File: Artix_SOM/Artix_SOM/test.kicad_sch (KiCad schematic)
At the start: 1 part

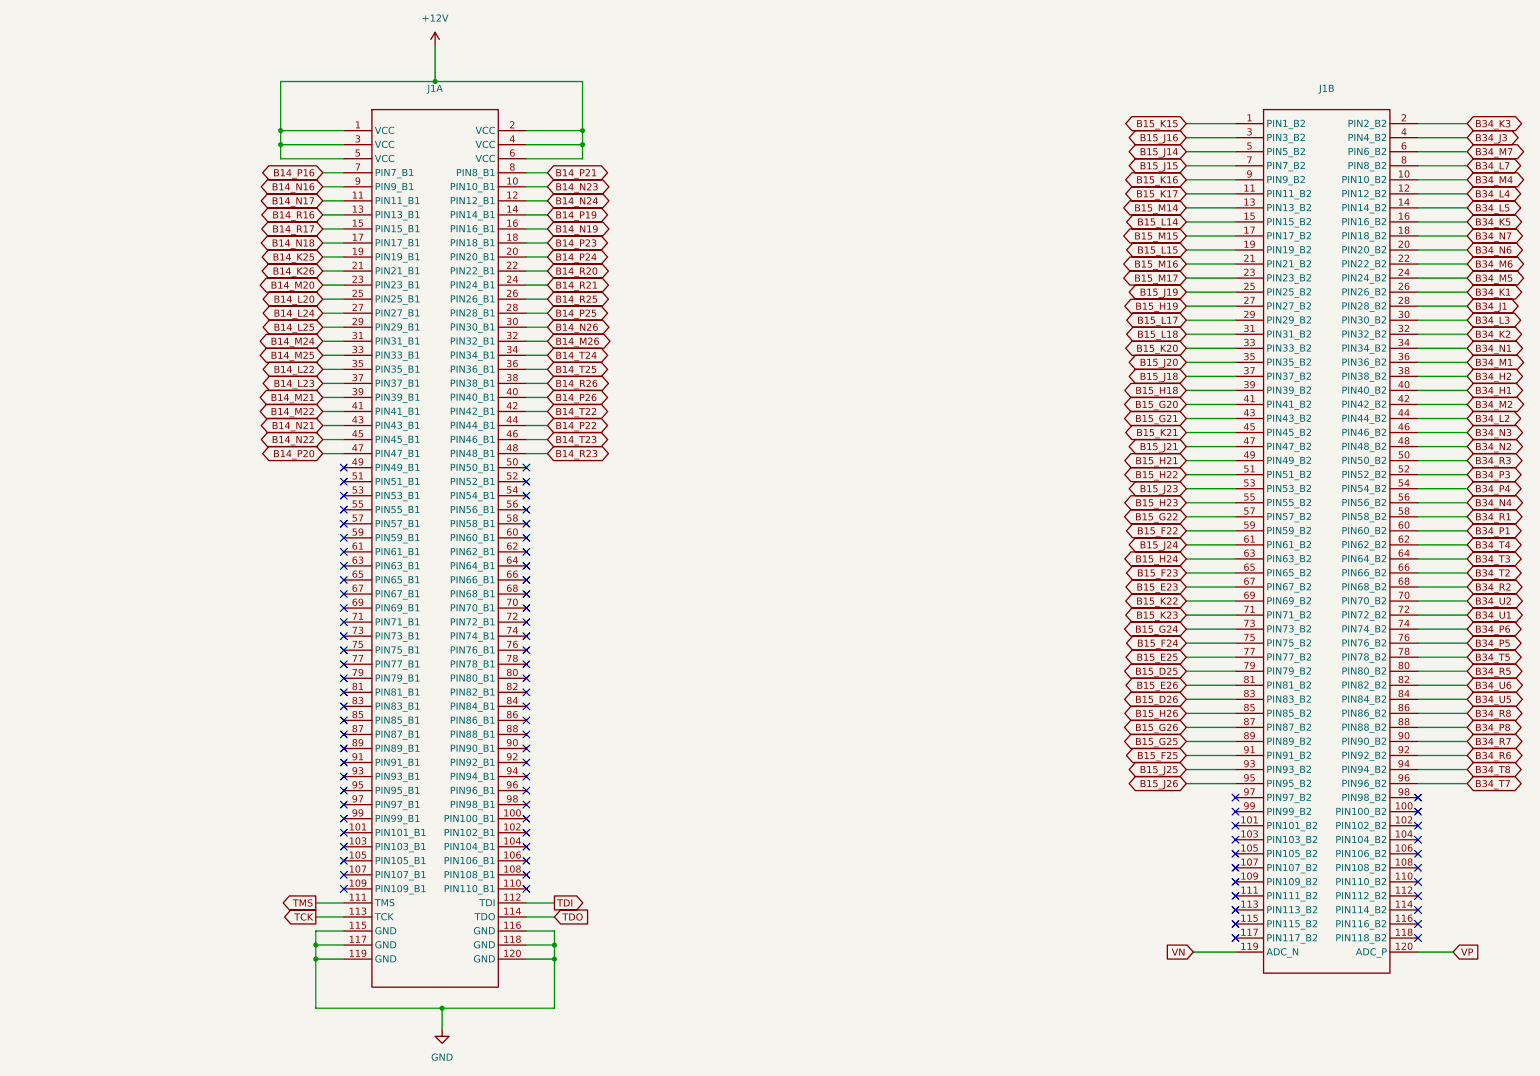
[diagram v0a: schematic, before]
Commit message: update
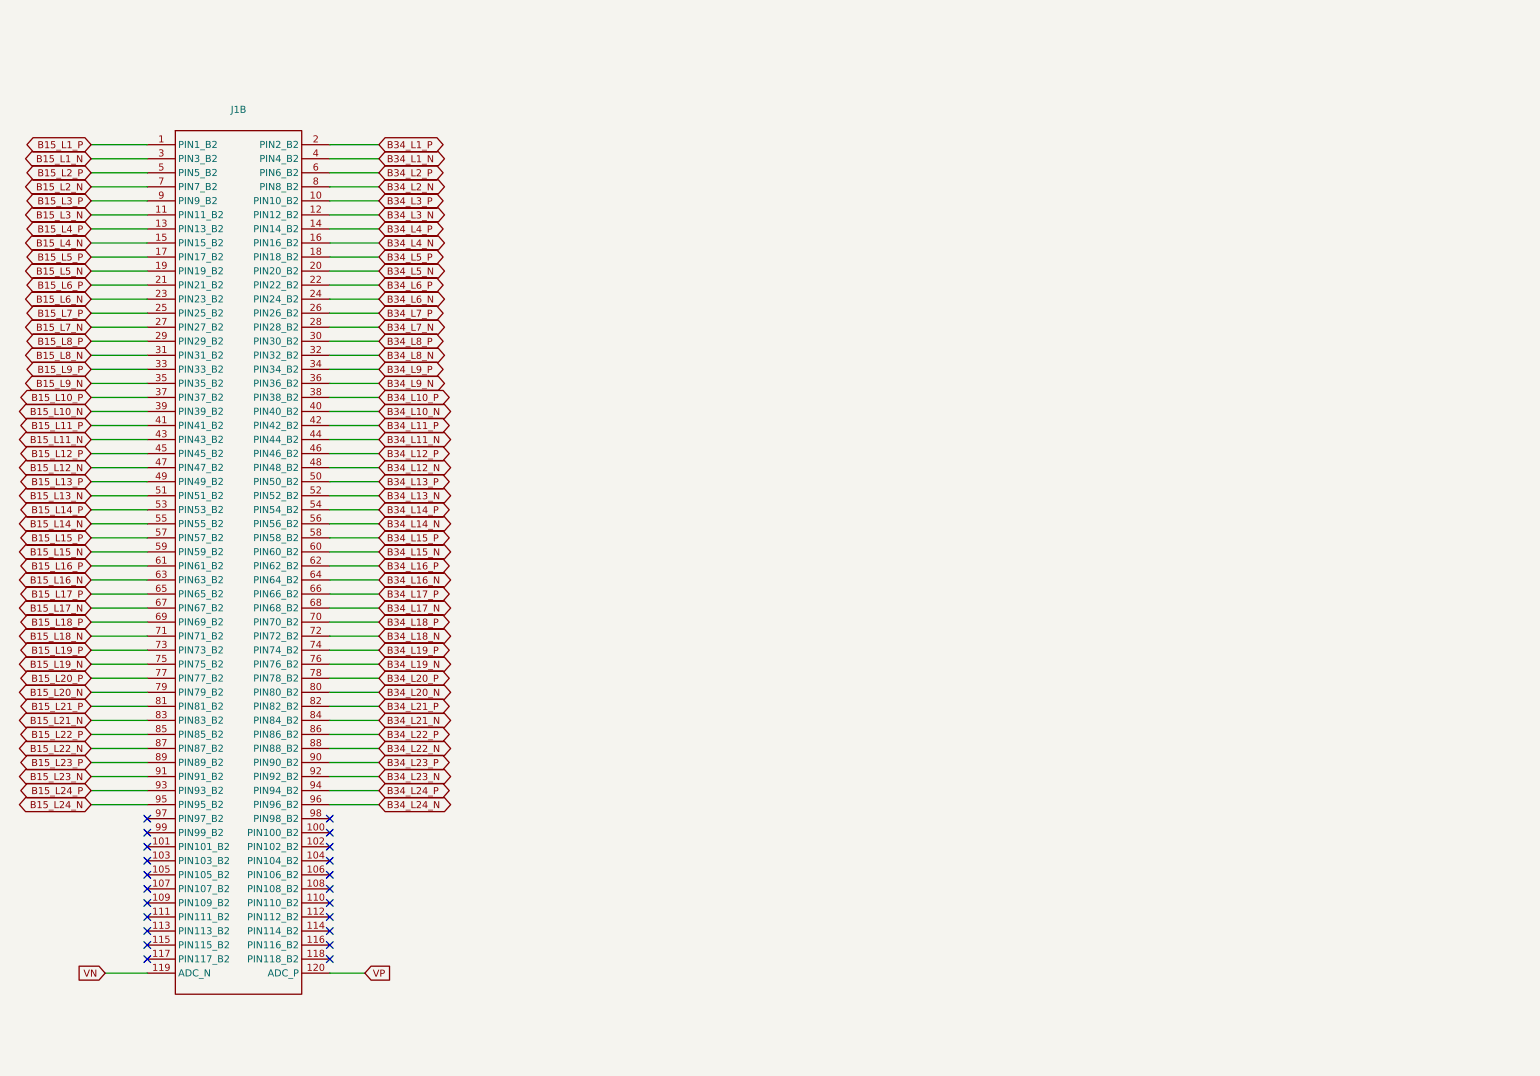
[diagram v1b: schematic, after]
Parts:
- removed unit 1 of J1
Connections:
- net B15_D25 renamed B15_L20_N
- net B15_D26 renamed B15_L21_N
- net B15_E23 renamed B15_L17_N
- net B15_E25 renamed B15_L20_P
- net B15_E26 renamed B15_L21_P
- net B15_F22 renamed B15_L15_N
- net B15_F23 renamed B15_L17_P
- net B15_F24 renamed B15_L19_N
- net B15_F25 renamed B15_L23_N
- net B15_G20 renamed B15_L11_P
- net B15_G21 renamed B15_L11_N
- net B15_G22 renamed B15_L15_P
- net B15_G24 renamed B15_L19_P
- net B15_G25 renamed B15_L23_P
- net B15_G26 renamed B15_L22_N
- net B15_H18 renamed B15_L10_N
- net B15_H19 renamed B15_L7_N
- net B15_H21 renamed B15_L13_P
- net B15_H22 renamed B15_L13_N
- net B15_H23 renamed B15_L14_N
- net B15_H24 renamed B15_L16_N
- net B15_H26 renamed B15_L22_P
- net B15_J14 renamed B15_L2_P
- net B15_J15 renamed B15_L2_N
- net B15_J16 renamed B15_L1_N
- net B15_J18 renamed B15_L10_P
- net B15_J19 renamed B15_L7_P
- net B15_J20 renamed B15_L9_N
- net B15_J21 renamed B15_L12_N
- net B15_J23 renamed B15_L14_P
- net B15_J24 renamed B15_L16_P
- net B15_J25 renamed B15_L24_P
- net B15_J26 renamed B15_L24_N
- net B15_K15 renamed B15_L1_P
- net B15_K16 renamed B15_L3_P
- net B15_K17 renamed B15_L3_N
- net B15_K20 renamed B15_L9_P
- net B15_K21 renamed B15_L12_P
- net B15_K22 renamed B15_L18_P
- net B15_K23 renamed B15_L18_N
- net B15_L14 renamed B15_L4_N
- net B15_L15 renamed B15_L5_N
- net B15_L17 renamed B15_L8_P
- net B15_L18 renamed B15_L8_N
- net B15_M14 renamed B15_L4_P
- net B15_M15 renamed B15_L5_P
- net B15_M16 renamed B15_L6_P
- net B15_M17 renamed B15_L6_N
- net B34_H1 renamed B34_L10_N
- net B34_H2 renamed B34_L10_P
- net B34_J1 renamed B34_L7_N
- net B34_J3 renamed B34_L1_N
- net B34_K1 renamed B34_L7_P
- net B34_K2 renamed B34_L8_N
- net B34_K3 renamed B34_L1_P
- net B34_K5 renamed B34_L4_N
- net B34_L2 renamed B34_L11_N
- net B34_L3 renamed B34_L8_P
- net B34_L4 renamed B34_L3_N
- net B34_L5 renamed B34_L4_P
- net B34_L7 renamed B34_L2_N
- net B34_M1 renamed B34_L9_N
- net B34_M2 renamed B34_L11_P
- net B34_M4 renamed B34_L3_P
- net B34_M5 renamed B34_L6_N
- net B34_M6 renamed B34_L6_P
- net B34_M7 renamed B34_L2_P
- net B34_N1 renamed B34_L9_P
- net B34_N2 renamed B34_L12_N
- net B34_N3 renamed B34_L12_P
- net B34_N4 renamed B34_L14_N
- net B34_N6 renamed B34_L5_N
- net B34_N7 renamed B34_L5_P
- net B34_P1 renamed B34_L15_N
- net B34_P3 renamed B34_L13_N
- net B34_P4 renamed B34_L14_P
- net B34_P5 renamed B34_L19_N
- net B34_P6 renamed B34_L19_P
- net B34_P8 renamed B34_L22_N
- net B34_R1 renamed B34_L15_P
- net B34_R2 renamed B34_L17_N
- net B34_R3 renamed B34_L13_P
- net B34_R5 renamed B34_L20_N
- net B34_R6 renamed B34_L23_N
- net B34_R7 renamed B34_L23_P
- net B34_R8 renamed B34_L22_P
- net B34_T2 renamed B34_L17_P
- net B34_T3 renamed B34_L16_N
- net B34_T4 renamed B34_L16_P
- net B34_T5 renamed B34_L20_P
- net B34_T7 renamed B34_L24_N
- net B34_T8 renamed B34_L24_P
- net B34_U1 renamed B34_L18_N
- net B34_U2 renamed B34_L18_P
- net B34_U5 renamed B34_L21_N
- net B34_U6 renamed B34_L21_P
- no-connect marks 84 -> 22
